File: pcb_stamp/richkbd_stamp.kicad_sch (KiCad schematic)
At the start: 48 parts, among them J1 USB_C_Receptacle, J2 OLED, K0 key-diode-led, K1 key-diode-led, K10 key-diode-led, K100 key-diode-led, K101 key-diode-led, K102 key-diode-led, K11 key-diode-led, K110 key-diode-led, K111 key-diode-led, K112 key-diode-led, K12 key-diode-led, K2 key-diode-led, K20 key-diode-led, K21 key-diode-led, K22 key-diode-led, K30 key-diode-led, K31 key-diode-led, K32 key-diode-led, K33 key-diode-led, K40 key-diode-led, K41 key-diode-led, K42 key-diode-led, K43 key-diode-led, K50 key-diode-led, K51 key-diode-led, K52 key-diode-led, K53 key-diode-led, K60 key-diode-led, K61 key-diode-led, K62 key-diode-led, K63 key-diode-led, K70 key-diode-led, K71 key-diode-led, K72 key-diode-led, K73 key-diode-led, K80 key-diode-led, K81 key-diode-led, K82 key-diode-led, K83 key-diode-led, K90 key-diode-led, K91 key-diode-led, K92 key-diode-led, U1 RP2040_Stamp

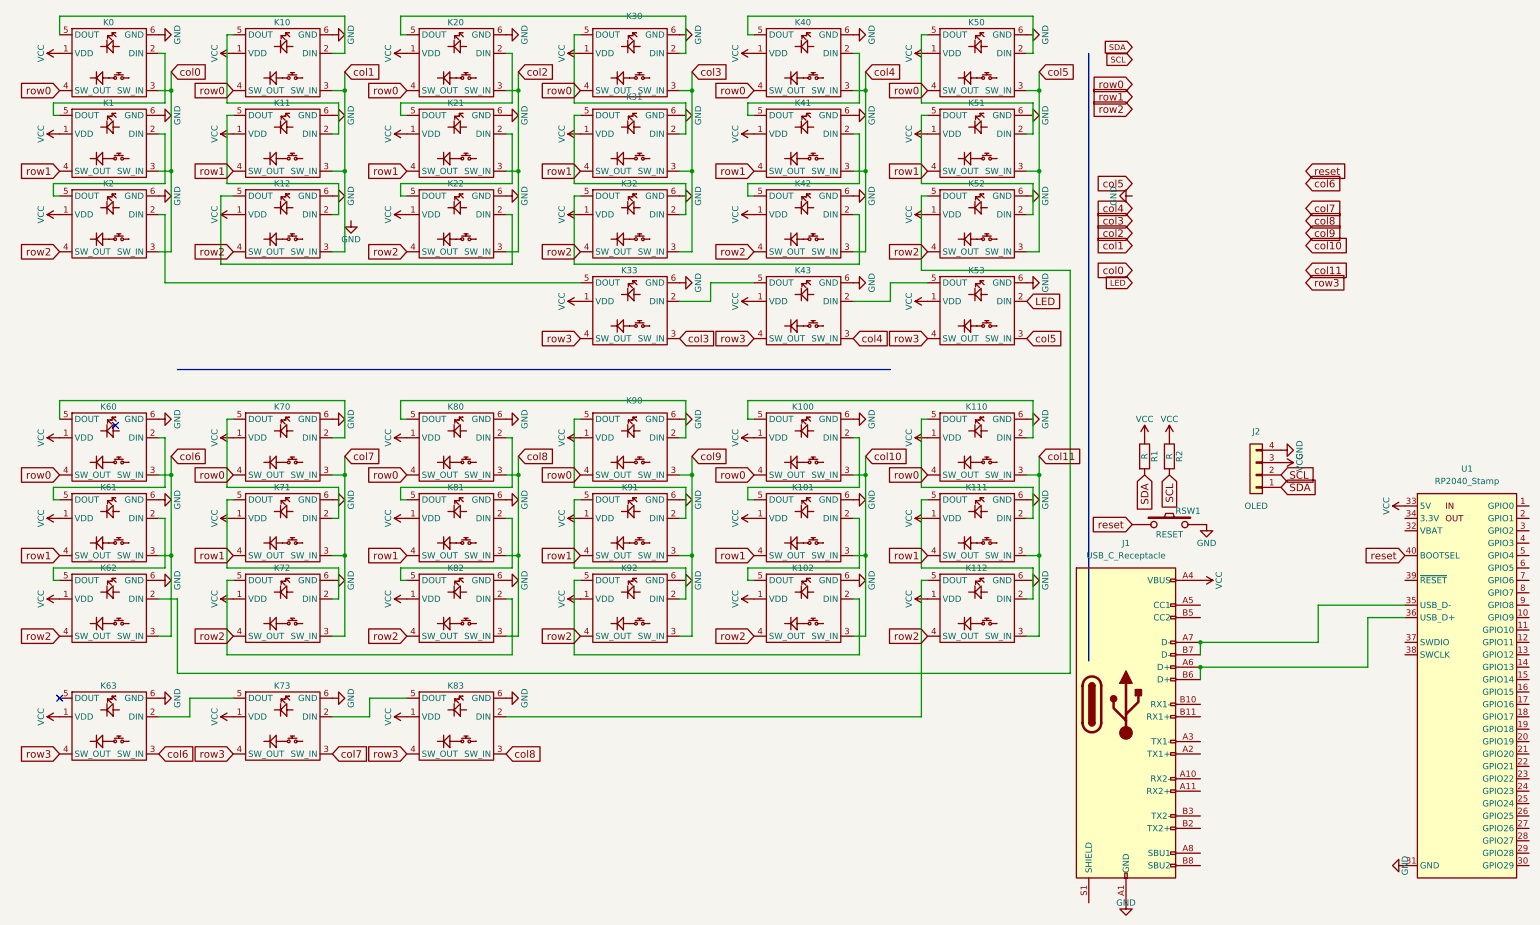
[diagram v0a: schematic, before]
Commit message: Finished stamp routing
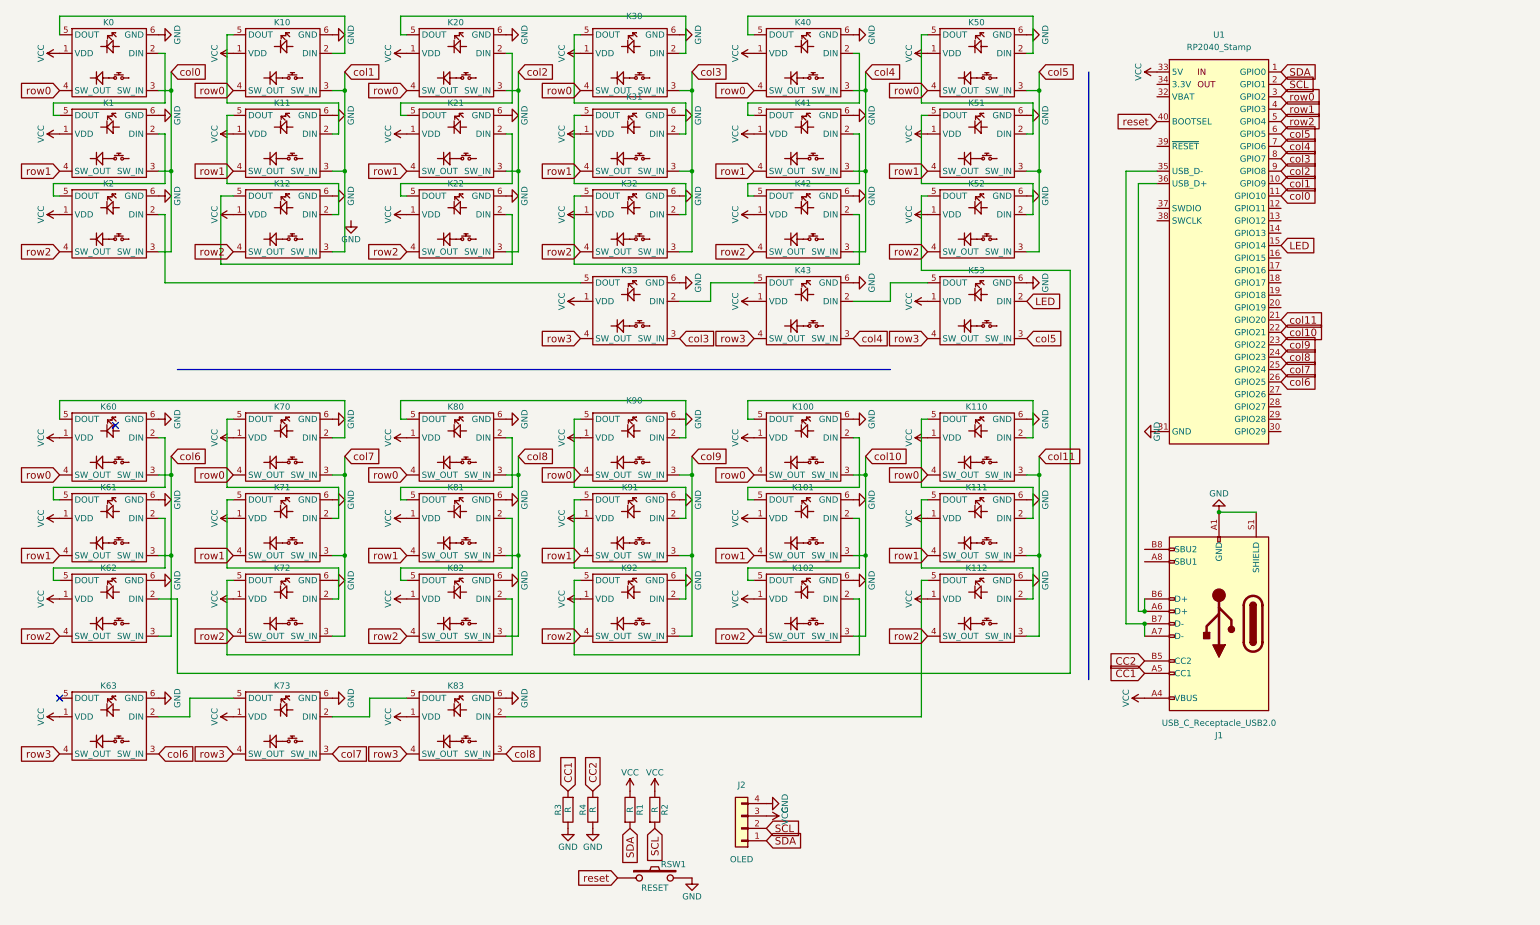
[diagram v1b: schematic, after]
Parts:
- removed J1: USB_C_Receptacle, symbol Connector:USB_C_Receptacle
- added J1: USB_C_Receptacle_USB2.0, Connector_USB:USB_C_Receptacle_GCT_USB4085, symbol Connector:USB_C_Receptacle_USB2.0
- added R3, R4: R, Resistor_SMD:R_0805_2012Metric, symbol Device:R
- R1, R2: footprint kbd:R -> Resistor_SMD:R_0805_2012Metric
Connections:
- net GND: now also J1.A1 (GND), J1.A12 (GND), J1.B1 (GND), J1.B12 (GND), J1.S1 (SHIELD), R3.1, R4.1
- net LED: now also U1.15 (GPIO14)
- net SCL: now also U1.2 (GPIO1)
- net SDA: now also U1.1 (GPIO0)
- net VCC: now also J1.A4 (VBUS), J1.A9 (VBUS), J1.B4 (VBUS), J1.B9 (VBUS)
- net col0: now also U1.11 (GPIO10)
- net col1: now also U1.10 (GPIO9)
- net col10: now also U1.22 (GPIO21)
- net col11: now also U1.21 (GPIO20)
- net col2: now also U1.9 (GPIO8)
- net col3: now also U1.8 (GPIO7)
- net col4: now also U1.7 (GPIO6)
- net col5: now also U1.6 (GPIO5)
- net col6: now also U1.26 (GPIO25)
- net col7: now also U1.25 (GPIO24)
- net col8: now also U1.24 (GPIO23)
- net col9: now also U1.23 (GPIO22)
- net row0: now also U1.3 (GPIO2)
- net row1: now also U1.4 (GPIO3)
- net row2: now also U1.5 (GPIO4)
- net at U1.36 (USB_D+): now also J1.A6 (D+), J1.B6 (D+)
- net at U1.35 (USB_D-): now also J1.A7 (D-), J1.B7 (D-)
- new net CC1: J1.A5 (CC1), R3.2
- new net CC2: J1.B5 (CC2), R4.2
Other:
- moved on the sheet: J2, R1, R2, RSW1, U1
